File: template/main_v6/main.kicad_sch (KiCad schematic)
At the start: 15 parts

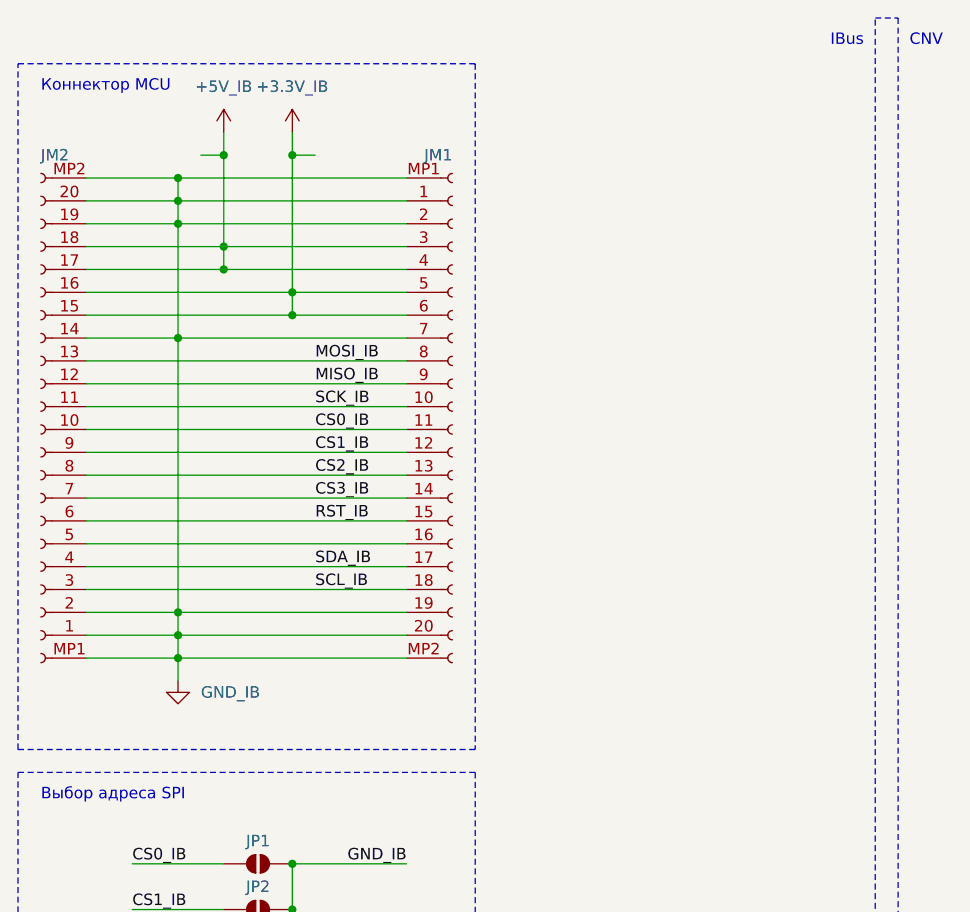
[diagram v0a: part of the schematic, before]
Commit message: new structure
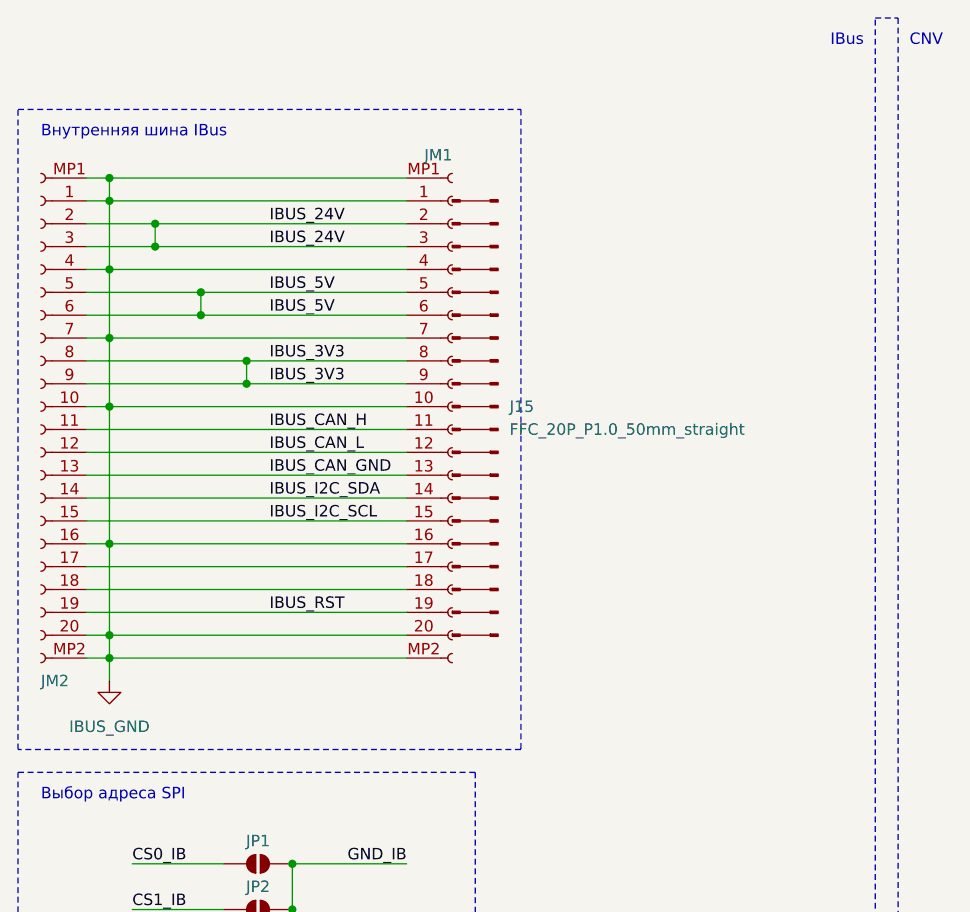
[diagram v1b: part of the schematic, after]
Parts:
- removed JM2: AFA07-S20FCC-00, kicad_inventree_lib:AFA11-S20GLA-00, symbol kicad_inventree_lib:AFA11-S20GLA-00
- added J15: FFC_20P_P1.0_50mm_straight, symbol kicad_inventree_lib:FFC_20P_P1.0_50mm_straight
- added JM2: AFA07-S20FCC-00, kicad_inventree_lib:AFA07S20FCA00, symbol kicad_inventree_lib:AFA07-S20FCC-00
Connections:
- net MOSI_IB is gone; now on net IBUS_3V3: JM1.8 (Pin_8)
- net SCK_IB is gone; now on net IBUS_GND: JM1.10 (Pin_10)
- net +3.3V_IB: no longer JM1.5 (Pin_5), JM1.6 (Pin_6)
- net CS0_IB: no longer JM1.11 (Pin_11)
- net CS1_IB: no longer JM1.12 (Pin_11)
- net CS2_IB: no longer JM1.13 (Pin_11)
- net CS3_IB: no longer JM1.14 (Pin_11)
- net GND_IB: no longer JM1.1 (Pin_1), JM1.19 (Pin_11), JM1.2 (Pin_2), JM1.20 (Pin_11), JM1.7 (Pin_7), JM1.MP1 (Pin_11), JM1.MP2 (Pin_11)
- net IBUS_GND: now reaches JM1.16 (Pin_11)
- net IBUS_GND: now also JM1.1 (Pin_1), JM1.20 (Pin_11), JM1.4 (Pin_4), JM1.7 (Pin_7), JM1.MP1 (Pin_11), JM1.MP2 (Pin_11), JM2.1 (Pin_1), JM2.10 (Pin_10), JM2.16 (Pin_11), JM2.20 (Pin_11), JM2.4 (Pin_4), JM2.7 (Pin_7), JM2.MP1 (Pin_11), JM2.MP2 (Pin_11)
- net +5V_IB renamed IBUS_24V
- net IBUS_24V: now also JM1.2 (Pin_2), JM2.2 (Pin_2), JM2.3 (Pin_3); no longer JM1.4 (Pin_4)
- net MISO_IB renamed IBUS_3V3
- net IBUS_3V3: now also JM2.8 (Pin_8), JM2.9 (Pin_9)
- net RST_IB renamed IBUS_I2C_SCL
- net IBUS_I2C_SCL: now also JM2.15 (Pin_11)
- net SCL_IB: no longer names the net of JM1.18 (Pin_11)
- net SCL_IB: now also JM2.18 (Pin_11)
- net SDA_IB: no longer names the net of JM1.17 (Pin_11)
- net SDA_IB: now also JM2.17 (Pin_11)
- new net IBUS_5V: JM1.5 (Pin_5), JM1.6 (Pin_6), JM2.5 (Pin_5), JM2.6 (Pin_6)
- new net IBUS_CAN_GND: JM1.13 (Pin_11), JM2.13 (Pin_11)
- new net IBUS_CAN_H: JM1.11 (Pin_11), JM2.11 (Pin_11)
- new net IBUS_CAN_L: JM1.12 (Pin_11), JM2.12 (Pin_11)
- new net IBUS_I2C_SDA: JM1.14 (Pin_11), JM2.14 (Pin_11)
- new net IBUS_RST: JM1.19 (Pin_11), JM2.19 (Pin_11)
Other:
- note added: "Внутренняя шина IBus"
- note removed: "Коннектор MCU"
